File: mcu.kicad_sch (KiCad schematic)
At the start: 3 parts, among them J1 FTSH-105-01-F-DV-P-TR, U1 nRF52840

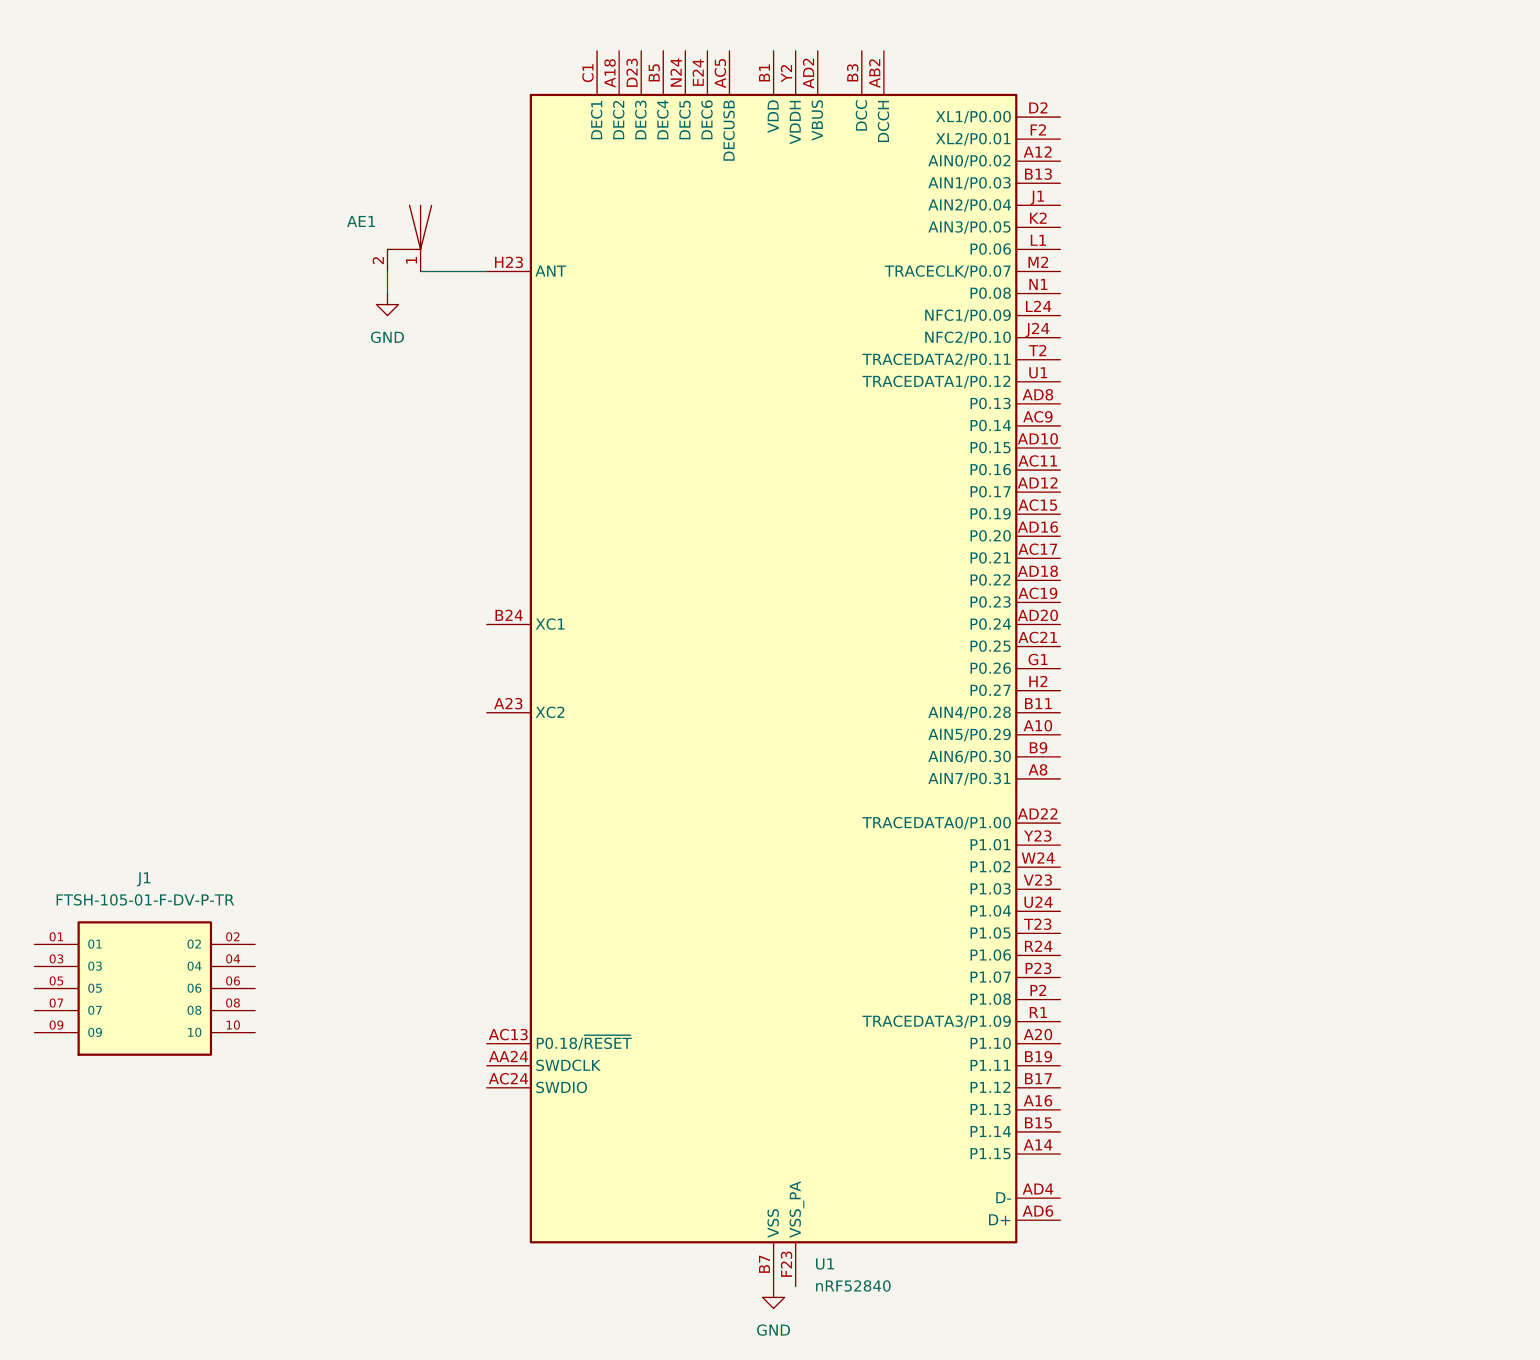
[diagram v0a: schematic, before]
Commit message: Setup charging
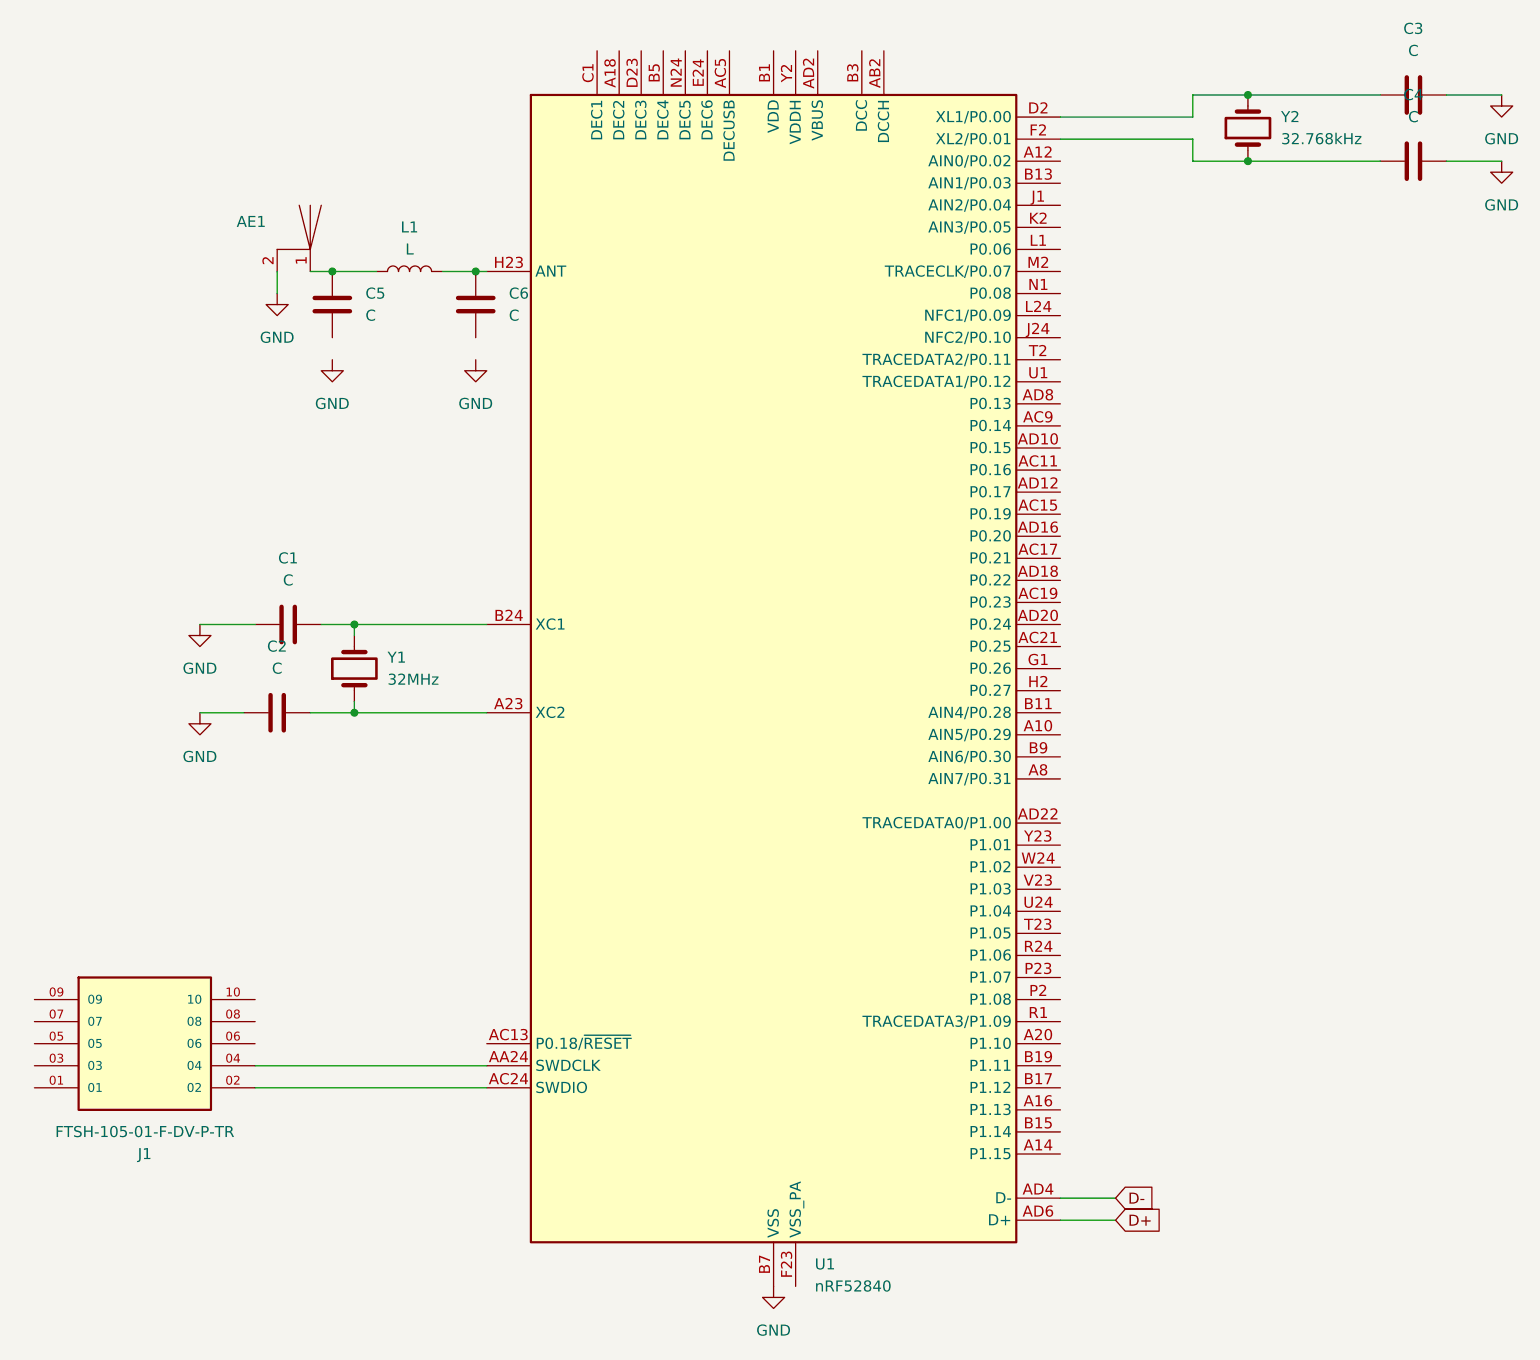
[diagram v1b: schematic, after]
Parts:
- added C1, C2, C3, C4, C5, C6: C, symbol Device:C
- added L1: L, symbol Device:L
- added Y1: 32MHz, Crystal:Crystal_SMD_HC49-SD, symbol Device:Crystal
- added Y2: 32.768kHz, Crystal:Crystal_SMD_3215-2Pin_3.2x1.5mm, symbol Device:Crystal
- J1: LCSC PN (none) -> C5136979; Part Number (none) -> FTSH-105-01-F-DV-P-TR
- U1: LCSC PN (none) -> C190794; Part Number (none) -> NRF52840-QIAA-R
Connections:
- net GND: now also C1.1, C2.1, C3.2, C4.2
- net at J1.02: now also U1.AC24 (SWDIO)
- net at J1.04: now also U1.AA24 (SWDCLK)
- net at U1.A23 (XC2): now also C2.2, Y1.1
- net D-: now reaches U1.AD4 (D-)
- net D+: now reaches U1.AD6 (D+)
- net at U1.B24 (XC1): now also C1.2, Y1.2
- net at U1.D2 (XL1/P0.00): now also C3.1, Y2.2
- net at U1.F2 (XL2/P0.01): now also C4.1, Y2.1
- net at AE1.1: now also C5.1, L1.1; no longer U1.H23 (ANT)
- new net: C6.1, L1.2, U1.H23 (ANT)
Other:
- moved on the sheet: AE1, J1
